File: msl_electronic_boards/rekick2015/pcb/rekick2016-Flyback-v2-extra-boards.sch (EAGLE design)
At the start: 14 parts, among them J3 79109-12, P1 87759-12, Q1 PSMN7R8-120PS, Q2 PSMN7R8-120PS, X1 79109-12, X2 87832-04

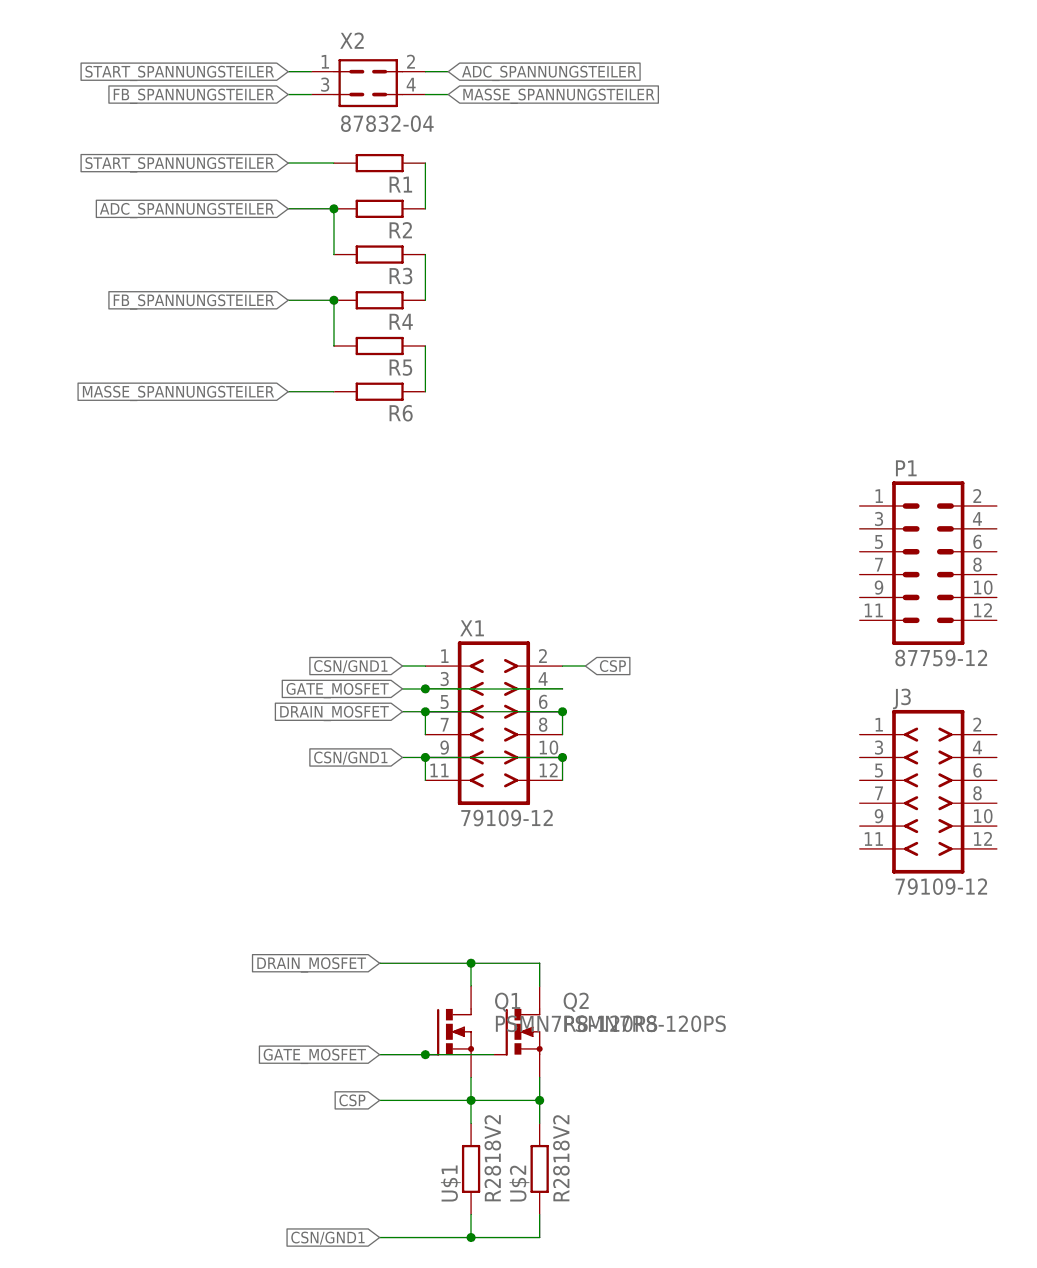
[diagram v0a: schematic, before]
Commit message: rekick 2016 + extra boards
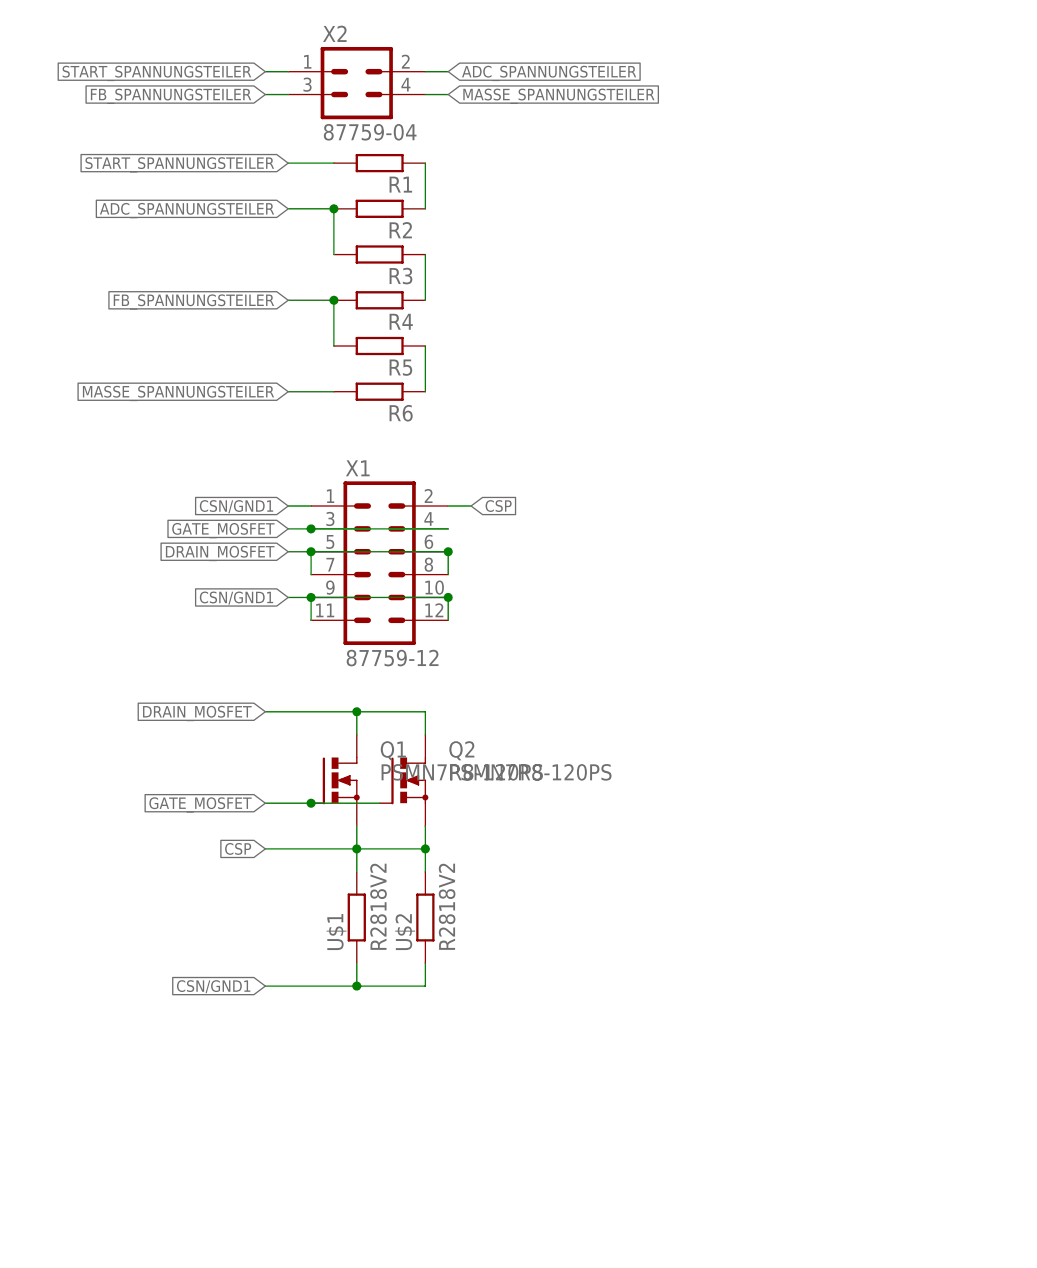
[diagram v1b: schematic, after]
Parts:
- removed J3: 79109-12, con-molex-milli-grid:79109-12
- removed P1: 87759-12, con-molex-milli-grid:87759-12
- X1: value 79109-12 -> 87759-12; device con-molex-milli-grid:79109-12 -> con-molex-milli-grid:87759-12
- X2: value 87832-04 -> 87759-04; device con-molex:87832-04 -> con-molex-milli-grid:87759-04
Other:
- moved on the sheet: Q1, Q2, U$1, U$2
